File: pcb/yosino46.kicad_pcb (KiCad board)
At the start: 2 copper layers, 156.9 x 115 mm, 90 parts, among them J0 LED, J1 TRRS, J2 OLED, J3 OLED, J4 OLED, SW1 SW_PUSH, SW10 SW_PUSH, SW11 SW_PUSH, SW12 SW_PUSH, SW13 SW_PUSH, SW14 SW_PUSH, SW15 SW_PUSH, SW16 SW_PUSH, SW17 SW_PUSH, SW18 SW_PUSH, SW19 SW_PUSH, SW2 SW_PUSH, SW20 SW_PUSH, SW21 SW_PUSH, SW22 SW_PUSH, SW23 SW_PUSH, SW3 SW_PUSH, SW4 SW_PUSH, SW5 SW_PUSH, SW6 SW_PUSH, SW7 SW_PUSH, SW8 SW_PUSH, SW9 SW_PUSH, U1 ProMicro, U2 ProMicro

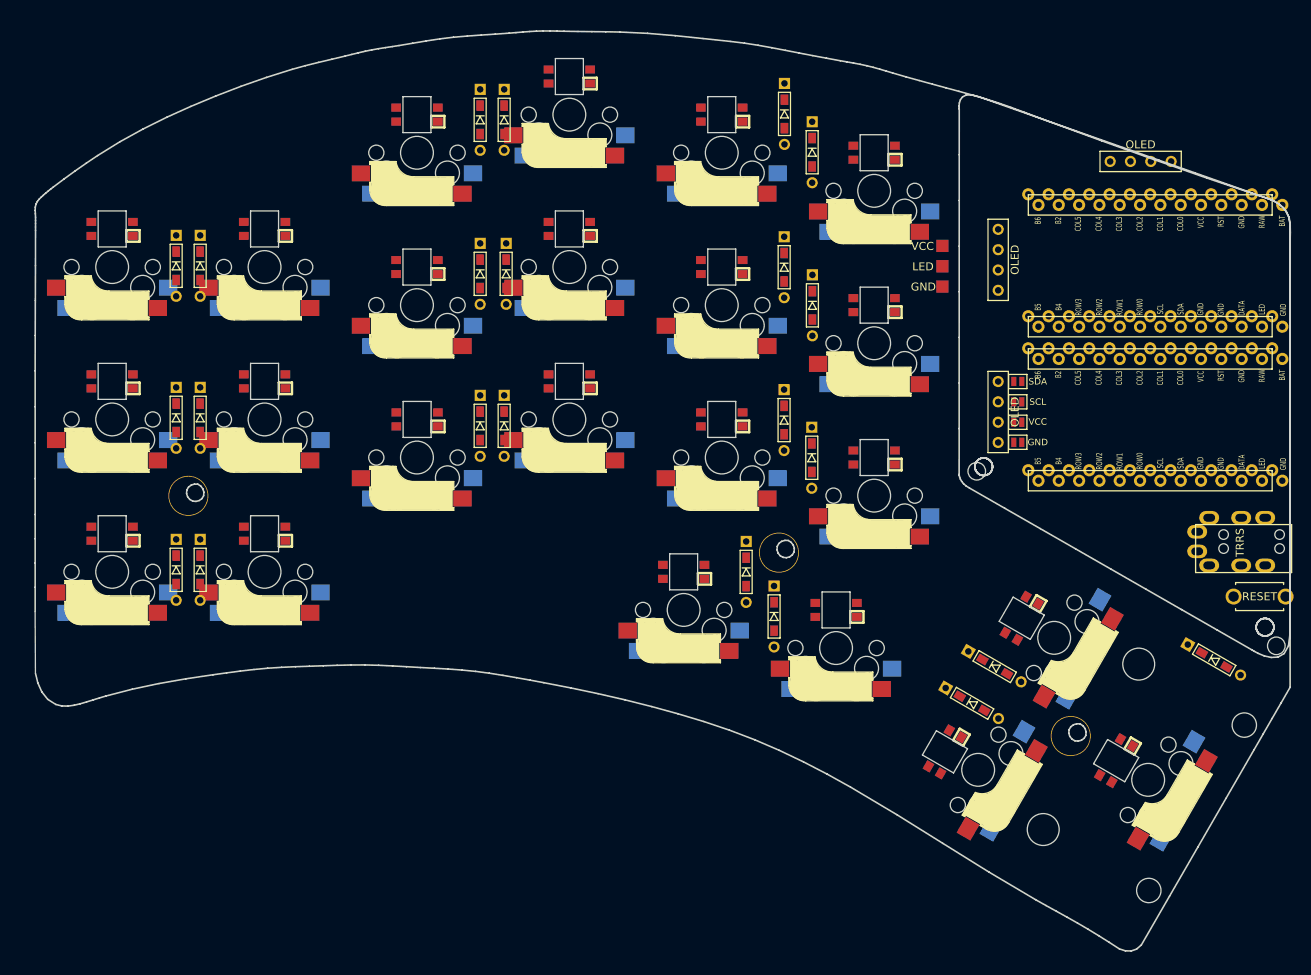
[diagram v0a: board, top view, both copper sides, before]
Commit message: yosino46作成
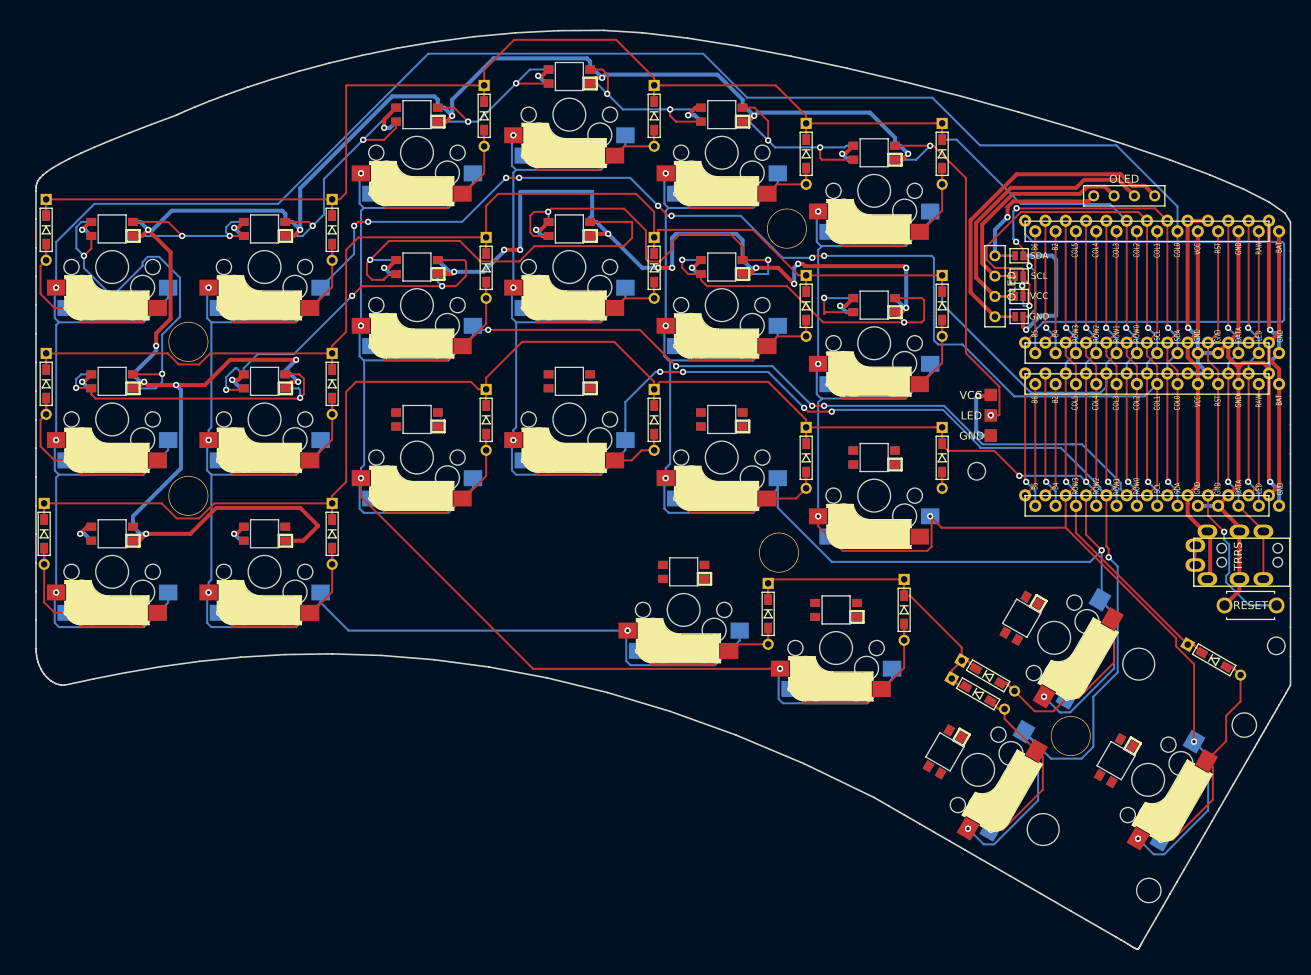
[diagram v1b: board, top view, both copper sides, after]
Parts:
- removed J2: OLED, yosino46:OLED
- added Ref**: Val**, yosino46:spacer, F.Cu at (60.0, 80.8)
- added Ref**: Val**, yosino46:spacer, F.Cu at (134.8, 66.6)
- L1, L10, L11, L12, L13, L14, L15, L16, L17, L18, L19, L2, L20, L21, L22, L23, L3, L4, L5, L6, L7, L8, L9: footprint yosino46:SK6812MINI_rev -> yosino46:SK6812MINI_padin_rev
- moved J0 19.6 mm to (160.3, 92.5)
- moved D16 18.8 mm to (118.2, 90.5)
- moved D4 18.8 mm to (118.2, 52.5)
- moved D10 18.5 mm to (118.2, 71.5)
- moved D13 17.1 mm to (42.0, 104.8)
- moved D14 17.1 mm to (78.0, 104.8)
- moved D2 17.1 mm to (78.0, 66.8)
- moved D8 17.0 mm to (78.0, 86.0)
- moved D1 16.9 mm to (42.2, 66.8)
- moved D7 16.8 mm to (42.2, 86.0)
- moved D18 16.3 mm to (154.2, 95.2)
- moved D20 16.3 mm to (149.5, 114.2)
- moved D6 16.3 mm to (154.2, 57.2)
- moved D12 16.2 mm to (154.2, 76.2)
- moved JP7 15.7 mm to (163.9, 75.1)
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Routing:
- net VCC: track 0.00 -> 396.5 mm, vias 0 -> 25
- net col1: track 0.00 -> 317.8 mm, vias 0 -> 12
- net col2: track 0.00 -> 302.3 mm, vias 0 -> 8
- net col0: track 0.00 -> 293.3 mm, vias 0 -> 3
- net col3: track 0.00 -> 265.2 mm, vias 0 -> 9
- net row1: track 0.00 -> 227.7 mm, vias 0 -> 2
- net row0: track 0.00 -> 223.6 mm, vias 0 -> 2
- net row2: track 0.00 -> 219.1 mm, vias 0 -> 3
- net col4: track 0.00 -> 209.5 mm, vias 0 -> 5
- net col5: track 0.00 -> 203.1 mm, vias 0 -> 6
- net GND: track 0.00 -> 192.9 mm, vias 0 -> 18
- net row3: track 0.00 -> 113.1 mm, vias 0 -> 2
- net LED: track 0.00 -> 85.4 mm, vias 0 -> 4
- net Net-(U2-Pad12): track 0.00 -> 78.6 mm
- net SCL: track 0.00 -> 73.0 mm, vias 0 -> 3
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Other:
- board size 156.9 x 115 mm -> 156.8 x 114.8 mm

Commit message: yosino46作成
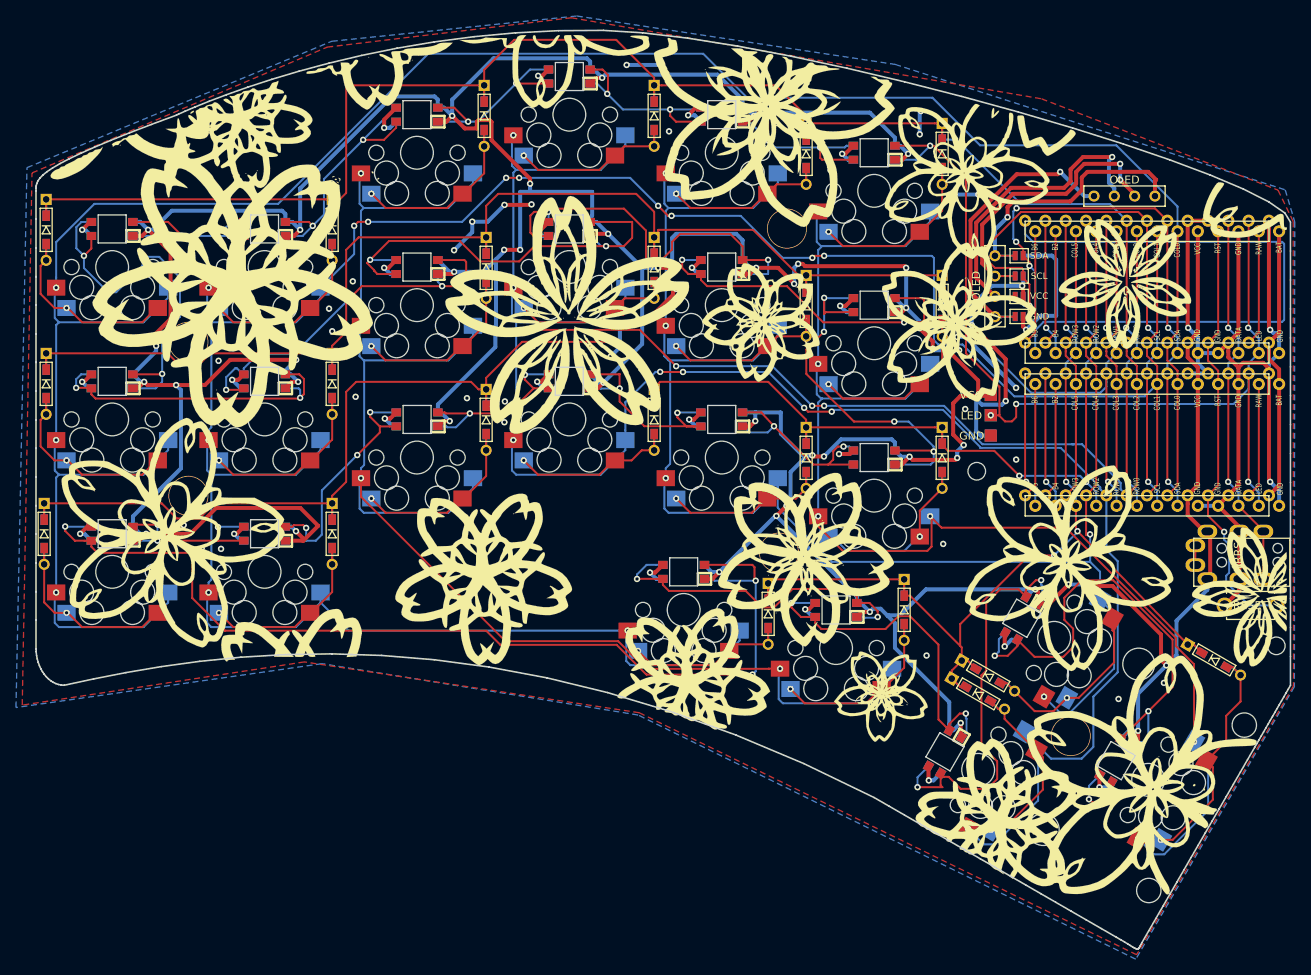
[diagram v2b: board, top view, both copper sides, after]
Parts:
- added G***: LOGO, yosino46:sakura_rev, F.Cu at (123.8, 96.8)
- added G***: LOGO, yosino46:sakura, F.Cu at (123.8, 96.8)
- L1, L10, L11, L12, L13, L14, L15, L16, L17, L18, L19, L2, L20, L21, L22, L23, L3, L4, L5, L6, L7, L8, L9: footprint yosino46:SK6812MINI_padin_rev -> yosino46:SK6812MINI_rev
- moved J4 7.65 mm to (180.8, 62.5), turned to 180 degrees
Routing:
- net VCC: track 396.5 -> 695.0 mm, vias 25 -> 50
- net Net-(L13-Pad1): track 0.00 -> 127.5 mm, vias 0 -> 3
- net GND: track 192.9 -> 270.3 mm, vias 18 -> 64
- net Net-(L22-Pad1): track 0.00 -> 60.8 mm, vias 0 -> 2
- net Net-(L21-Pad1): track 0.00 -> 52.1 mm, vias 0 -> 2
- net Net-(L20-Pad1): track 0.00 -> 43.6 mm, vias 0 -> 2
- net Net-(L19-Pad1): track 0.00 -> 42.2 mm, vias 0 -> 2
- net Net-(L12-Pad1): track 9.40 -> 51.3 mm, vias 1 -> 4
- net LED: track 85.4 -> 121.5 mm, vias 4 -> 5
- net Net-(L14-Pad3): track 0.00 -> 33.4 mm, vias 0 -> 3
- net Net-(L16-Pad3): track 0.00 -> 28.4 mm, vias 0 -> 2
- net Net-(L17-Pad3): track 0.00 -> 26.0 mm, vias 0 -> 2
- net Net-(L15-Pad3): track 0.00 -> 25.1 mm, vias 0 -> 2
- net Net-(L13-Pad3): track 0.00 -> 24.0 mm, vias 0 -> 3
- net row3: track 113.1 -> 135.6 mm, vias 2 -> 4
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- added copper zone on B.Cu, net GND
- added copper zone on F.Cu, net GND
